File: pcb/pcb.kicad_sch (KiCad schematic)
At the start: 3 parts

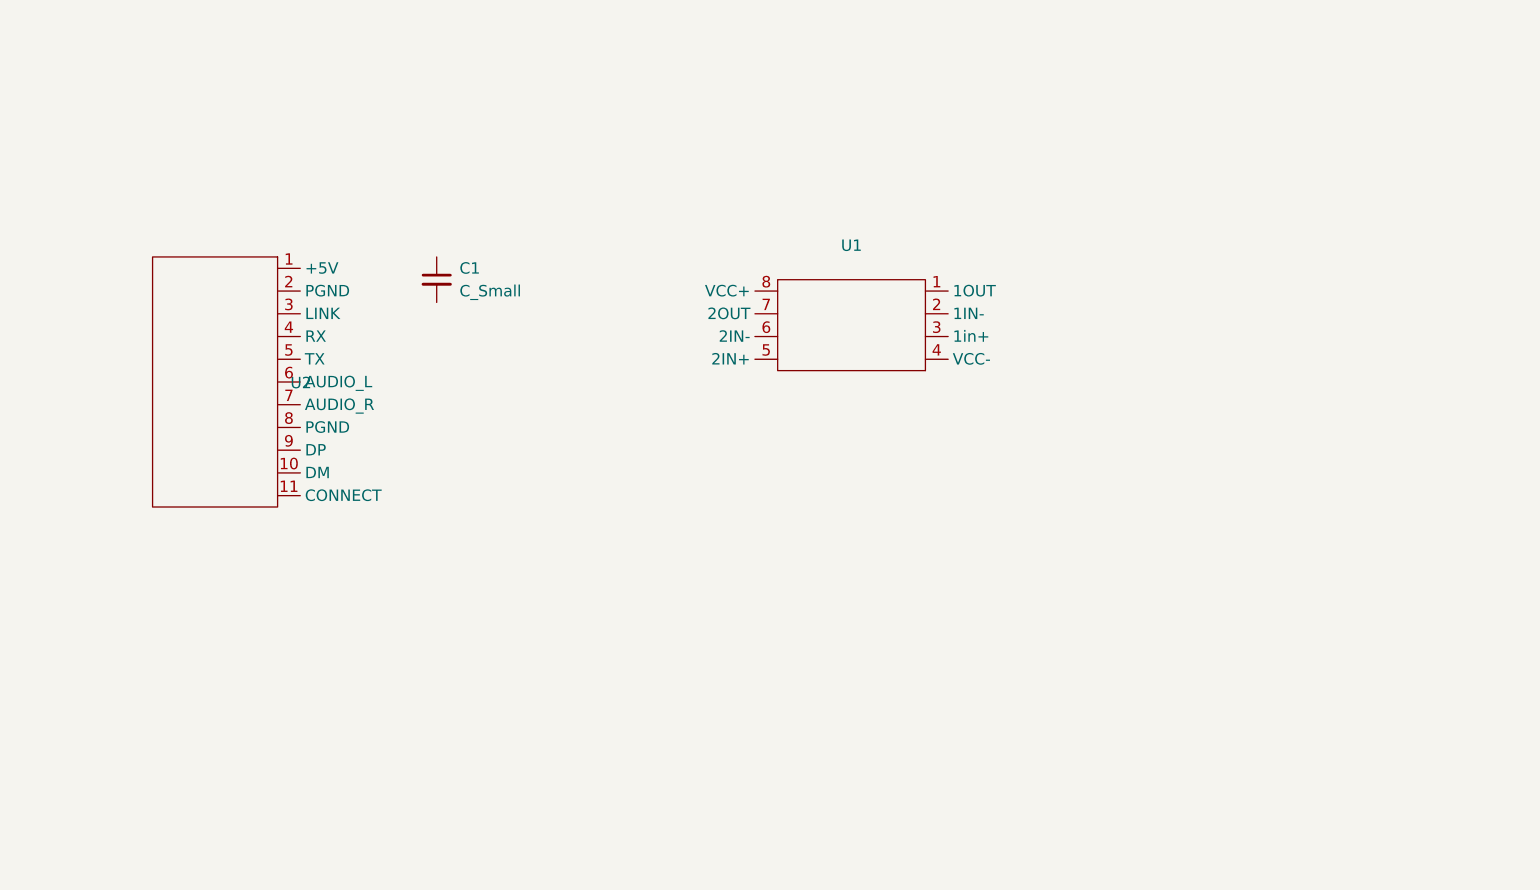
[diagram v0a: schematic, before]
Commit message: schematic v1
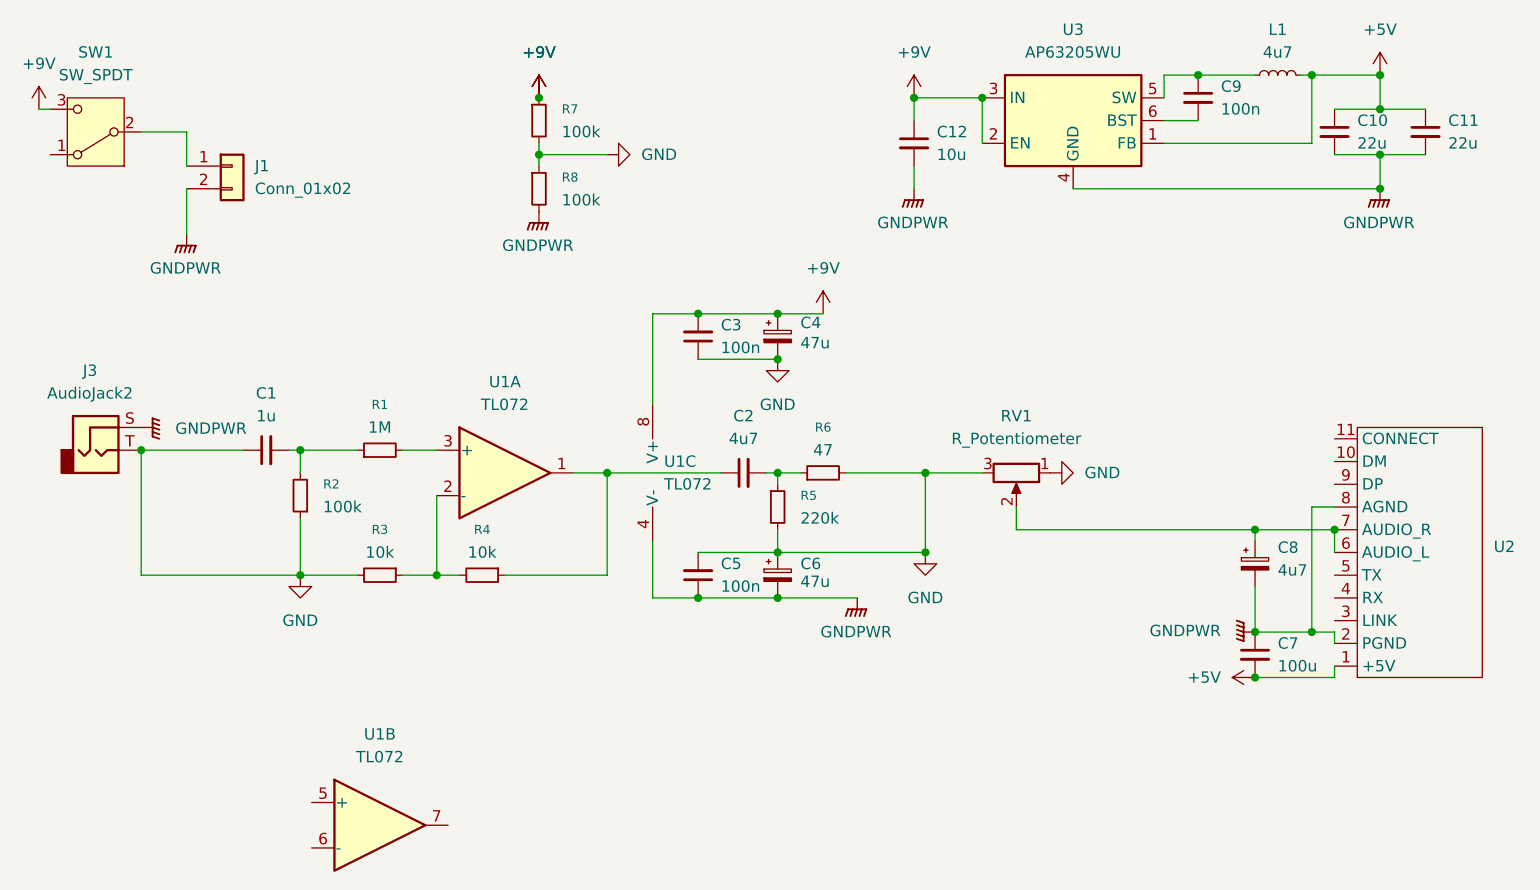
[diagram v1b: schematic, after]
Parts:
- removed U1: ~, symbol VoltLibrary:TL072
- added C10, C11: 22u, symbol Device:C_Small
- added C12: 10u, symbol Device:C_Small
- added C2: 4u7, symbol Device:C_Small
- added C3, C5, C9: 100n, symbol Device:C_Small
- added C4, C6: 47u, symbol Device:C_Polarized_Small
- added C7: 100u, symbol Device:C_Small
- added C8: 4u7, symbol Device:C_Polarized_Small
- added J1: Conn_01x02, symbol Connector_Generic:Conn_01x02
- added J3: AudioJack2, symbol Connector_Audio:AudioJack2
- added L1: 4u7, symbol Device:L_Small
- added R1: 1M, symbol Device:R_Small
- added R2, R7, R8: 100k, symbol Device:R_Small
- added R3, R4: 10k, symbol Device:R_Small
- added R5: 220k, symbol Device:R_Small
- added R6: 47, symbol Device:R_Small
- added RV1: R_Potentiometer, symbol Device:R_Potentiometer
- added SW1: SW_SPDT, symbol Switch:SW_SPDT
- added U1: TL072, symbol Amplifier_Operational:TL072
- added U3: AP63205WU, Package_TO_SOT_SMD:TSOT-23-6, symbol Regulator_Switching:AP63205WU
- C1: value C_Small -> 1u
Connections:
- net +5V: now reaches U2.1 (+5V)
- net +5V: now also C10.1, C11.1, C7.2, L1.2, U3.1 (FB)
- net GNDPWR: now reaches U2.2 (PGND)
- net GNDPWR: now also U2.8 (AGND), C10.2, C11.2, C12.2, C5.1, C6.2, C7.1, C8.2, J1.2 (Pin_2), J3.S, R8.2, U1.4 (V-), U3.4 (GND)
- net at U2.6 (AUDIO_L): now also U2.7 (AUDIO_R), C8.1, RV1.2
- net GND: now reaches C1.1
- net GND: now also C3.1, C4.2, C5.2, C6.1, J3.T, R2.1, R3.2, R5.2, R6.2, R7.2, R8.1, RV1.1, RV1.3
- net at C1.2: now also R1.1, R2.2
- new net: J1.1 (Pin_1), SW1.2 (B)
- new net: C9.1, L1.1, U3.5 (SW)
- new net: C9.2, U3.6 (BST)
- new net: C2.1, R4.1, U1.1
- new net: R3.1, R4.2, U1.2 (-)
- new net: R1.2, U1.3 (+)
- new net: C2.2, R5.1, R6.1
- new net +9V: C12.1, C3.2, C4.1, R7.1, SW1.3 (C), U1.8 (V+), U3.2 (EN), U3.3 (IN)
